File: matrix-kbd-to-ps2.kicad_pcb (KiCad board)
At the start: 2 copper layers, 33.9 x 39.4 mm, 14 parts, among them J1 CN13-CN14, J2 PS/2 - Mini-Din6, U1 PIC24FJ64GB002, U2 AMS1117

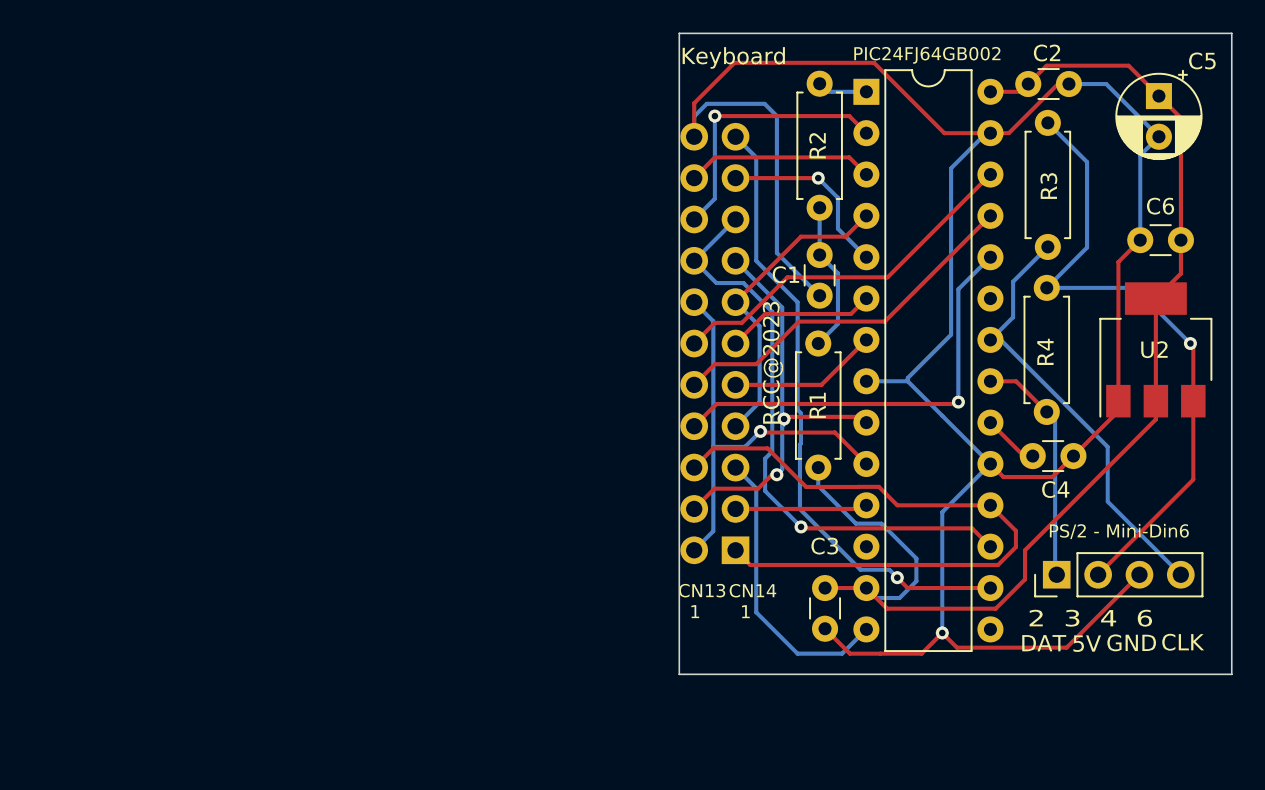
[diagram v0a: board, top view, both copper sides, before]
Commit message: Revision 1
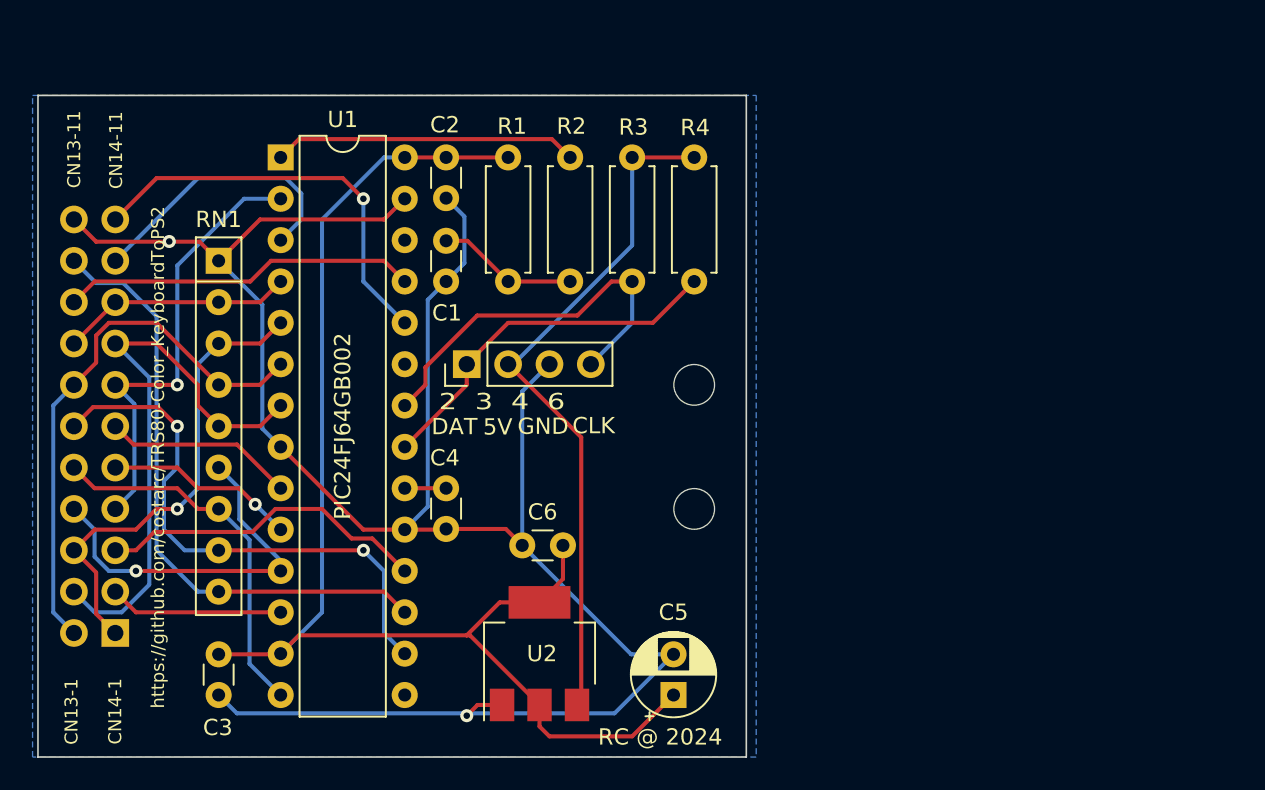
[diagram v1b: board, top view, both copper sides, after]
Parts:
- added H1: MountingHole, MountingHole:MountingHole_2.5mm, F.Cu at (80.0, 67.3)
- added H2: MountingHole, MountingHole:MountingHole_2.5mm, F.Cu at (80.0, 74.9)
- added RN1: 10K, Resistor_THT:R_Array_SIP9, F.Cu at (50.8, 59.7)
- moved C5 47.4 mm to (78.7, 86.4), turned to 90 degrees
- moved C6 42.3 mm to (69.4, 77.2)
- moved U2 42.2 mm to (70.5, 83.8)
- moved C2 38.9 mm to (64.8, 55.8), turned to 90 degrees
- moved C4 38.8 mm to (64.8, 76.2), turned to 90 degrees
- moved J2 38.5 mm to (66.0, 66.0)
- moved J1 38.4 mm to (44.5, 82.5)
- moved C3 37.5 mm to (50.8, 86.4)
- moved U1 36.2 mm to (54.6, 53.3)
- moved R1 26.9 mm to (68.6, 53.3), turned to -90 degrees
- moved R3 25.6 mm to (76.2, 53.3)
- moved R4 23.1 mm to (80.0, 53.3)
- moved C1 23.0 mm to (64.8, 61.0)
- moved R2 16.0 mm to (72.4, 53.3)
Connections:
- U1 pad 10: CN13-1 -> CN14-5
- U1 pad 11: CN14-2 -> CN13-4
- U1 pad 12: CAPS -> CN14-2
- U1 pad 14: CN14-3 -> CN13-5
- U1 pad 16: CN14-11 -> CN13-6
- U1 pad 17: CN13-8 -> CN13-10
- U1 pad 18: CN13-3 -> CN14-3
- U1 pad 2: CN13-9 -> CN14-4
- U1 pad 24: CN13-4 -> CN14-11
- U1 pad 25: CN13-5 -> CN13-9
- U1 pad 26: CN13-6 -> CAPS
- U1 pad 3: CN13-10 -> CN14-10
- U1 pad 4: CN14-4 -> CN13-8
- U1 pad 5: CN14-10 -> CN13-3
- U1 pad 6: CN14-6 -> CN13-1
- U1 pad 7: CN14-5 -> CN13-2
- U1 pad 9: CN13-2 -> CN14-6
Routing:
- net CN13-10: track 11.5 -> 37.7 mm
- net CN13-8: track 36.1 -> 14.3 mm, vias 1 -> 0
- net Net-(U1-Vpp/~{MCLR}/RE3): track 2.54 -> 18.7 mm
- net CN14-11: track 38.4 -> 25.5 mm
- net CN13-11: track 145.2 -> 132.7 mm, vias 1 -> 2
- net CN13-3: track 41.4 -> 29.1 mm, vias 0 -> 1
- net CN13-6: track 22.7 -> 34.2 mm, vias 0 -> 2
- net CN13-2: track 25.9 -> 35.1 mm, vias 2 -> 0
- net VDD: track 73.9 -> 83.0 mm
- net CN14-4: track 19.1 -> 27.8 mm, vias 0 -> 1
- net KBD_DATA: track 14.5 -> 22.7 mm
- net CN13-1: track 27.2 -> 33.6 mm, vias 1 -> 0
- net CN14-10: track 11.2 -> 17.3 mm, vias 1 -> 0
- net CN13-9: track 16.7 -> 21.9 mm, vias 1 -> 0
- net VCC: track 39.1 -> 42.8 mm, vias 1 -> 0
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- added copper zone on B.Cu, net CN13-11
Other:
- board size 33.9 x 39.4 mm -> 43.5 x 40.6 mm
- board text added: "CN13-1"
- board text added: "CN13-11"
- board text added: "CN14-1"
- board text added: "CN14-11"
- board text added: "Compatible with TRS-80 Color keyboard"
- board text added: "RC @ 2024"
- board text removed: "CN13 1"
- board text removed: "CN14 1"
- board text removed: "Copatible with TRS-80 Color keyboard"
- board text removed: "Keyboard"
- board text removed: "RCC@2023"
